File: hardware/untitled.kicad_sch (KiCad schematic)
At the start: 4 parts

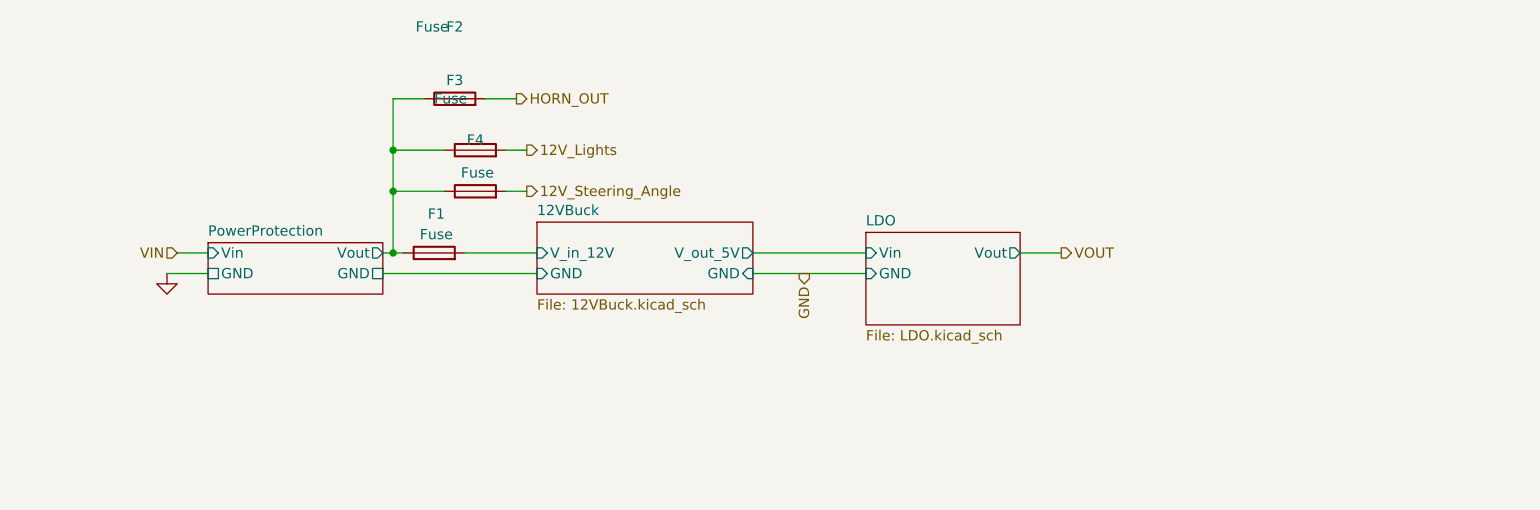
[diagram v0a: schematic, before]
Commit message: someone please check if i fucked up removing boot
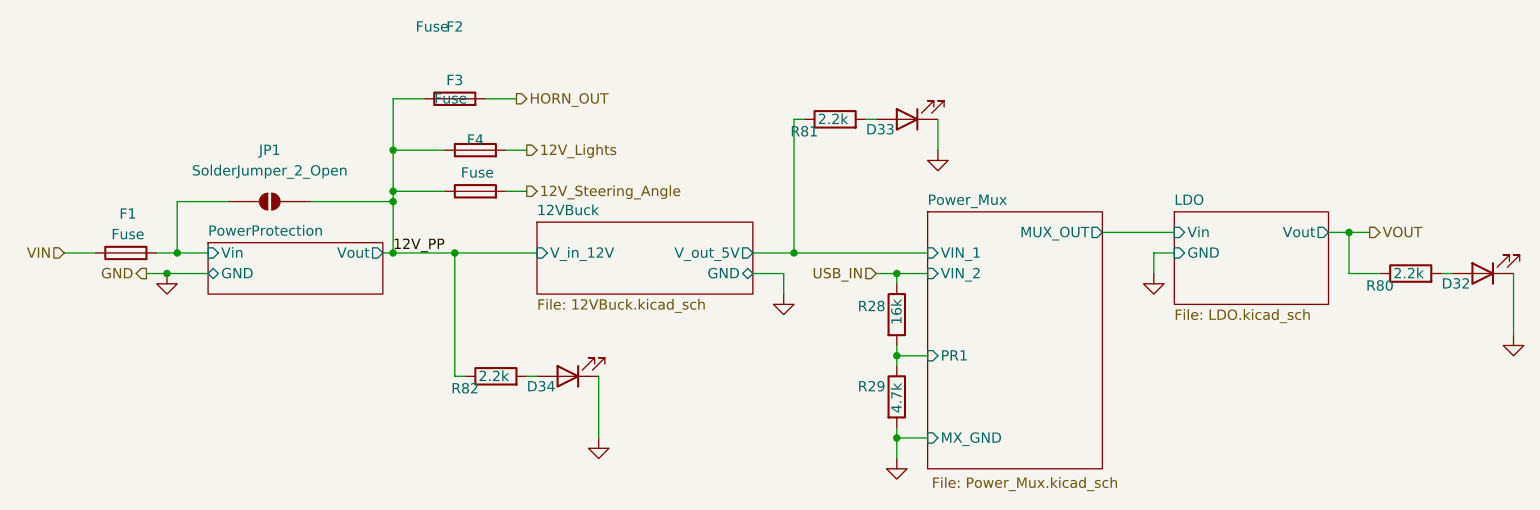
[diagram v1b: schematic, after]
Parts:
- added D32, D33, D34: Status LED, symbol Device:LED
- added JP1: SolderJumper_2_Open, symbol Jumper:SolderJumper_2_Open
- added R28: 16k, symbol Device:R
- added R29: 4.7k, symbol Device:R
- added R80, R81, R82: 2.2k, symbol Device:R
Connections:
- net 12VBuck/V_out_5V: now also R81.1
- net GND: now also D32.1 (K), D33.1 (K), D34.1 (K), R29.2
- net VIN: now also F1.1
- net VOUT: now also R80.1
- net 12VBuck/V_in_12V renamed PowerProtection/Vin
- net PowerProtection/Vin: now also JP1.1 (A)
- net PowerProtection/Vout renamed 12V_PP
- net 12V_PP: now also JP1.2 (B), R82.1; no longer F1.1
- new net: D33.2 (A), R81.2
- new net: D34.2 (A), R82.2
- new net: D32.2 (A), R80.2
- new net Power_Mux/PR1: R28.2, R29.1
- new net USB_IN: R28.1
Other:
- added sheet Power_Mux (Power_Mux.kicad_sch)
